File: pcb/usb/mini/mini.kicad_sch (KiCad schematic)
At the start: 2 parts, among them J1 USB_B_Mini, U1 CH340C

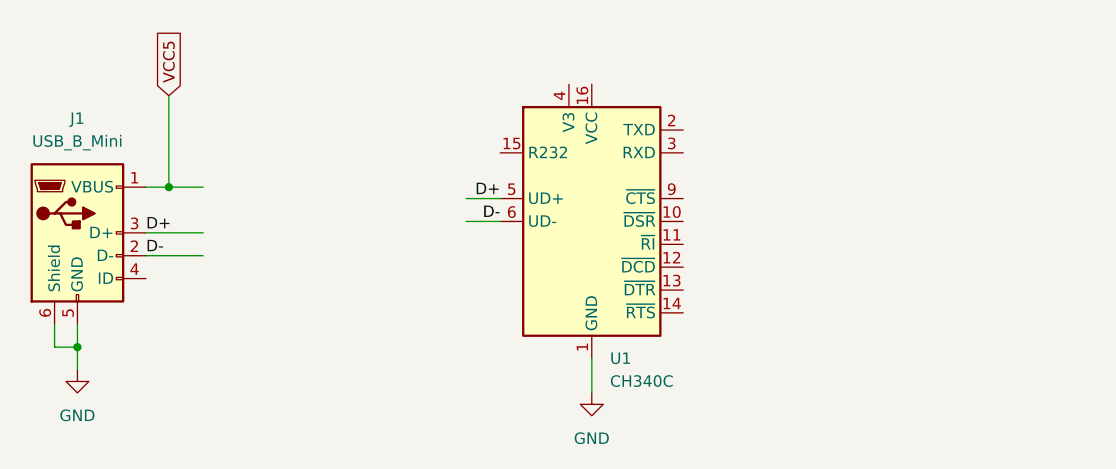
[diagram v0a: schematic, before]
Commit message: Signed-off-by: Dmitry Ponyatov <dponyatov@samsa.local>
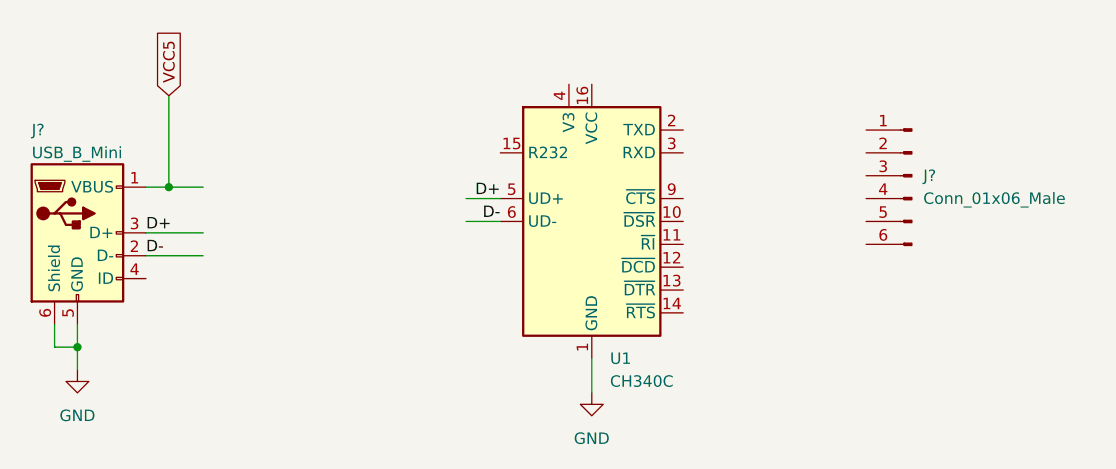
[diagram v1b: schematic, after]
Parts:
- added J?: Conn_01x06_Male, symbol Connector:Conn_01x06_Male
- J?: renamed from J1; symbol Connector:USB_B_Mini -> connector:USB_B_Mini
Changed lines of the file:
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@@
     )
+  )
+  (symbol (lib_id "Connector:Conn_01x06_Male") (at 175.26 82.55 0) (mirror y) (unit 1)
+    (in_bom yes) (on_board yes) (fields_autoplaced)
+    (property "Reference" "J?" (id 0) (at 176.53 82.5499 0)
+      (effects (font (size 1.27 1.27)) (justify right))
+    )
+    (property "Value" "Conn_01x06_Male" (id 1) (at 176.53 85.0899 0)
+      (effects (font (size 1.27 1.27)) (justify right))
+    )
+    (property "Footprint" "" (id 2) (at 175.26 82.55 0)
+      (effects (font (size 1.27 1.27)) hide)
+    )
+    (property "Datasheet" "~" (id 3) (at 175.26 82.55 0)
+      (effects (font (size 1.27 1.27)) hide)
+    )
+    (pin "1")
+    (pin "2")
+    (pin "3")
+    (pin "4")
+    (pin "5")
+    (pin "6")
   )
   (symbol (lib_id "power:GND") (at 139.7 106.68 0) (unit 1)
@@
     (pin "1")
   )
-  (symbol (lib_id "Connector:USB_B_Mini") (at 82.55 88.9 0) (unit 1)
+  (symbol (lib_id "connector:USB_B_Mini") (at 82.55 88.9 0) (unit 1)
     (in_bom yes) (on_board yes) (fields_autoplaced)
-    (property "Reference" "J1" (id 0) (at 82.55 76.2 0))
-    (property "Value" "USB_B_Mini" (id 1) (at 82.55 78.74 0))
+    (property "Reference" "J?" (id 0) (at 77.47 77.47 0)
+      (effects (font (size 1.27 1.27)) (justify left))
+    )
+    (property "Value" "USB_B_Mini" (id 1) (at 77.47 80.01 0)
+      (effects (font (size 1.27 1.27)) (justify left))
+    )
     (property "Footprint" "connector:USB_Mini-B_DS1104" (id 2) (at 86.36 90.17 0)
       (effects (font (size 1.27 1.27)) hide)
@@
       (reference "#PWR0102") (unit 1) (value "GND") (footprint "")
     )
+    (path "/aa0eaef1-e2de-4828-9cb9-7fe98fa29c67"
+      (reference "J?") (unit 1) (value "Conn_01x06_Male") (footprint "")
+    )
     (path "/ce1752a3-7b9b-4e5d-a7cf-dfe02fc97064"
-      (reference "J1") (unit 1) (value "USB_B_Mini") (footprint "connector:USB_Mini-B_DS1104")
+      (reference "J?") (unit 1) (value "USB_B_Mini") (footprint "connector:USB_Mini-B_DS1104")
     )
     (path "/e3c48a62-3601-400c-9094-a10797422302"
